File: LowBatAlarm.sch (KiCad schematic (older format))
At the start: 19 parts, among them J1 Battery, J2 Buzzer, Q1 BSN20, U1 ADCMP350, U2 ADP7142AUJZ

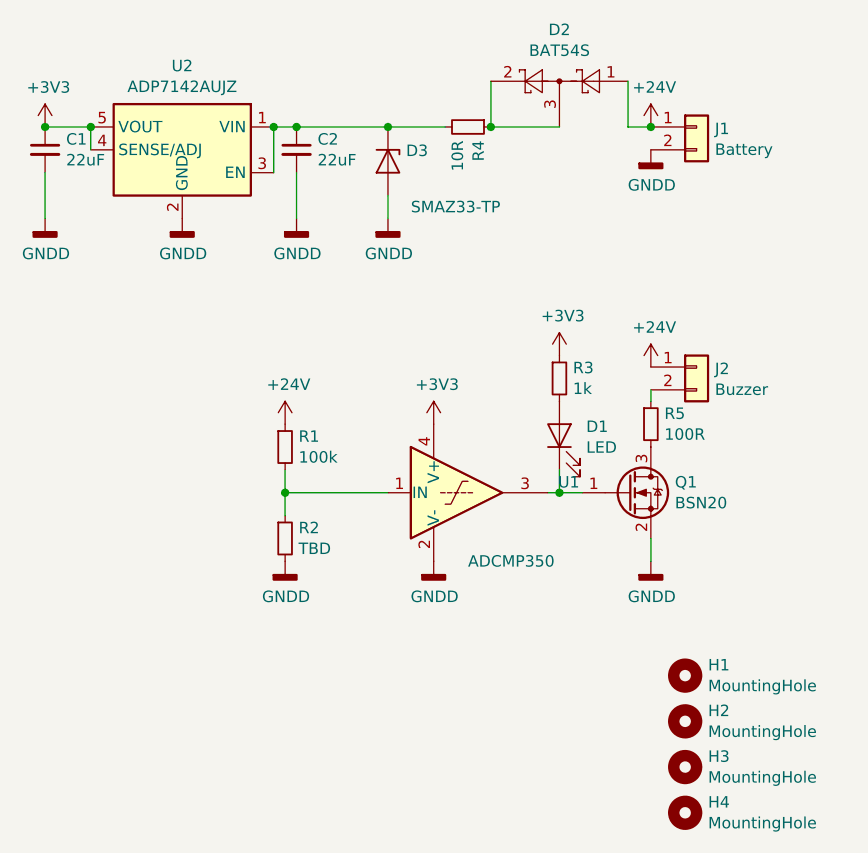
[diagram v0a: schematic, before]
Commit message: PCB opdatering
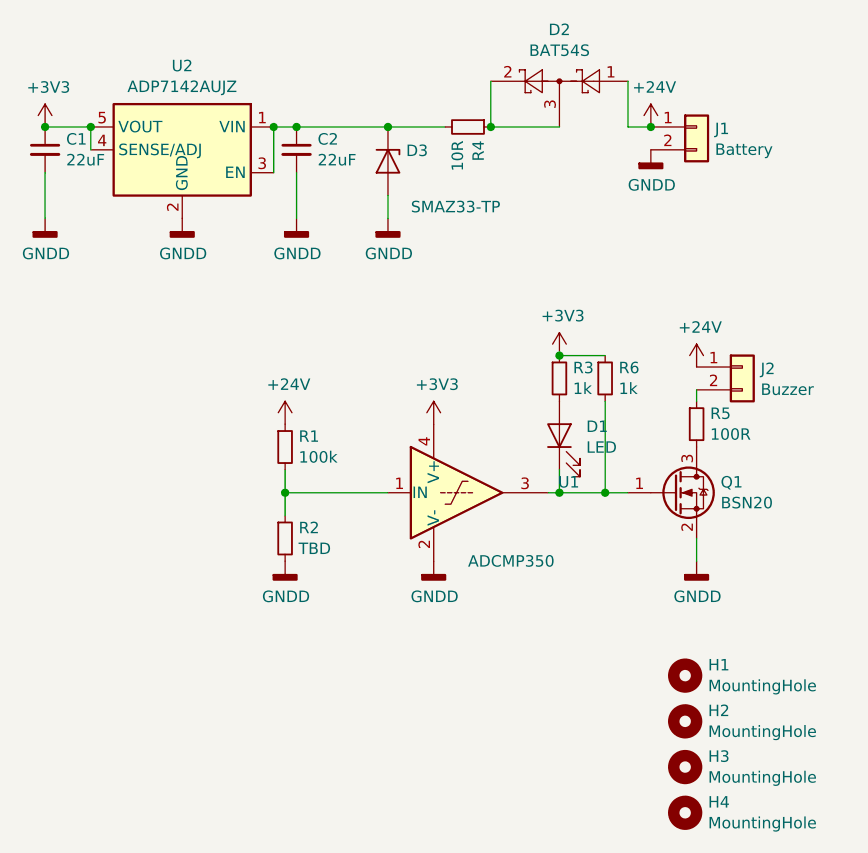
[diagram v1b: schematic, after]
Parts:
- added R6: 1k, Resistor_SMD:R_0805_2012Metric, symbol Device:R_Small
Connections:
- net +3V3: now also R6.1
- net at D1.1 (K), Q1.1 (G), U1.3: now also R6.2
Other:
- moved on the sheet: J2, Q1, R5
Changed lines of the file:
@@
 L Connector_Generic:Conn_01x02 J2
 U 1 1 5ED984DF
-P 7200 4000
-F 0 "J2" H 7280 3992 50  0000 L CNN
-F 1 "Buzzer" H 7280 3901 50  0000 L CNN
-F 2 "Connector_Molex:Molex_KK-254_AE-6410-02A_1x02_P2.54mm_Vertical" H 7200 4000 50  0001 C CNN
-F 3 "~" H 7200 4000 50  0001 C CNN
-	1    7200 4000
+P 7400 4000
+F 0 "J2" H 7480 3992 50  0000 L CNN
+F 1 "Buzzer" H 7480 3901 50  0000 L CNN
+F 2 "Connector_Molex:Molex_KK-254_AE-6410-02A_1x02_P2.54mm_Vertical" H 7400 4000 50  0001 C CNN
+F 3 "~" H 7400 4000 50  0001 C CNN
+	1    7400 4000
 	1    0    0    -1
 $EndComp
@@
 L power:+24V #PWR0106
 U 1 1 5ED9E892
-P 7000 4000
-F 0 "#PWR0106" H 7000 3850 50  0001 C CNN
-F 1 "+24V" H 7015 4173 50  0000 C CNN
-F 2 "" H 7000 4000 50  0001 C CNN
-F 3 "" H 7000 4000 50  0001 C CNN
-	1    7000 4000
+P 7200 4000
+F 0 "#PWR0106" H 7200 3850 50  0001 C CNN
+F 1 "+24V" H 7215 4173 50  0000 C CNN
+F 2 "" H 7200 4000 50  0001 C CNN
+F 3 "" H 7200 4000 50  0001 C CNN
+	1    7200 4000
 	1    0    0    -1
 $EndComp
@@
 L Transistor_FET:BSN20 Q1
 U 1 1 5ED9F4C0
-P 6900 4550
-F 0 "Q1" H 7105 4596 50  0000 L CNN
-F 1 "BSN20" H 7105 4505 50  0000 L CNN
-F 2 "Package_TO_SOT_SMD:SOT-23" H 7100 4475 50  0001 L CIN
-F 3 "http://www.diodes.com/assets/Datasheets/ds31898.pdf" H 6900 4550 50  0001 L CNN
-	1    6900 4550
+P 7100 4550
+F 0 "Q1" H 7305 4596 50  0000 L CNN
+F 1 "BSN20" H 7305 4505 50  0000 L CNN
+F 2 "Package_TO_SOT_SMD:SOT-23" H 7300 4475 50  0001 L CIN
+F 3 "http://www.diodes.com/assets/Datasheets/ds31898.pdf" H 7100 4550 50  0001 L CNN
+	1    7100 4550
 	1    0    0    -1
 $EndComp
@@
 L power:GNDD #PWR0107
 U 1 1 5EDA341D
-P 7000 4850
-F 0 "#PWR0107" H 7000 4600 50  0001 C CNN
-F 1 "GNDD" H 7004 4695 50  0000 C CNN
-F 2 "" H 7000 4850 50  0001 C CNN
-F 3 "" H 7000 4850 50  0001 C CNN
-	1    7000 4850
-	1    0    0    -1
-$EndComp
-Wire Wire Line
-	7000 4750 7000 4850
-Wire Wire Line
-	6700 4550 6600 4550
+P 7200 4850
+F 0 "#PWR0107" H 7200 4600 50  0001 C CNN
+F 1 "GNDD" H 7204 4695 50  0000 C CNN
+F 2 "" H 7200 4850 50  0001 C CNN
+F 3 "" H 7200 4850 50  0001 C CNN
+	1    7200 4850
+	1    0    0    -1
+$EndComp
+Wire Wire Line
+	7200 4750 7200 4850
 $Comp
 L power:+24V #PWR0108
@@
 L Device:R_Small R5
 U 1 1 5ED87ACF
-P 7000 4250
-F 0 "R5" H 7059 4296 50  0000 L CNN
-F 1 "100R" H 7059 4205 50  0000 L CNN
-F 2 "Resistor_SMD:R_0805_2012Metric" H 7000 4250 50  0001 C CNN
-F 3 "~" H 7000 4250 50  0001 C CNN
-	1    7000 4250
-	1    0    0    -1
-$EndComp
-Wire Wire Line
-	7000 4100 7000 4150
+P 7200 4250
+F 0 "R5" H 7259 4296 50  0000 L CNN
+F 1 "100R" H 7259 4205 50  0000 L CNN
+F 2 "Resistor_SMD:R_0805_2012Metric" H 7200 4250 50  0001 C CNN
+F 3 "~" H 7200 4250 50  0001 C CNN
+	1    7200 4250
+	1    0    0    -1
+$EndComp
+Wire Wire Line
+	7200 4100 7200 4150
+$Comp
+L Device:R_Small R6
+U 1 1 5EEA5E71
+P 6800 4050
+F 0 "R6" H 6859 4096 50  0000 L CNN
+F 1 "1k" H 6859 4005 50  0000 L CNN
+F 2 "Resistor_SMD:R_0805_2012Metric" H 6800 4050 50  0001 C CNN
+F 3 "~" H 6800 4050 50  0001 C CNN
+	1    6800 4050
+	1    0    0    -1
+$EndComp
+Wire Wire Line
+	6800 3950 6600 3950
+Connection ~ 6600 3950
+Wire Wire Line
+	6600 4550 6800 4550
+Wire Wire Line
+	6800 4150 6800 4550
+Connection ~ 6800 4550
+Wire Wire Line
+	6800 4550 6900 4550
 $EndSCHEMATC
